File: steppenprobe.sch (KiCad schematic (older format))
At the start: 85 parts, among them J1 USB_C_Receptacle_USB2.0, J2 Conn_ST_STDC14, J4 Conn_01x16, Q1 2N7002, SW1 SW_SPDT, SW2 SW_Push, U1 FT2232HL, U10 74LVC1G125, U11 74LVC1G125, U12 74LVC1G125, U2 XC6206PxxxMR, U3 SRV05-4, U4 93LCxxB, U5 74LVC1G125, U6 74LVC1G126, U7 74LVC1G125, U8 74LVC1G125, U9 74LVC1G125, Y1 Crystal_GND24

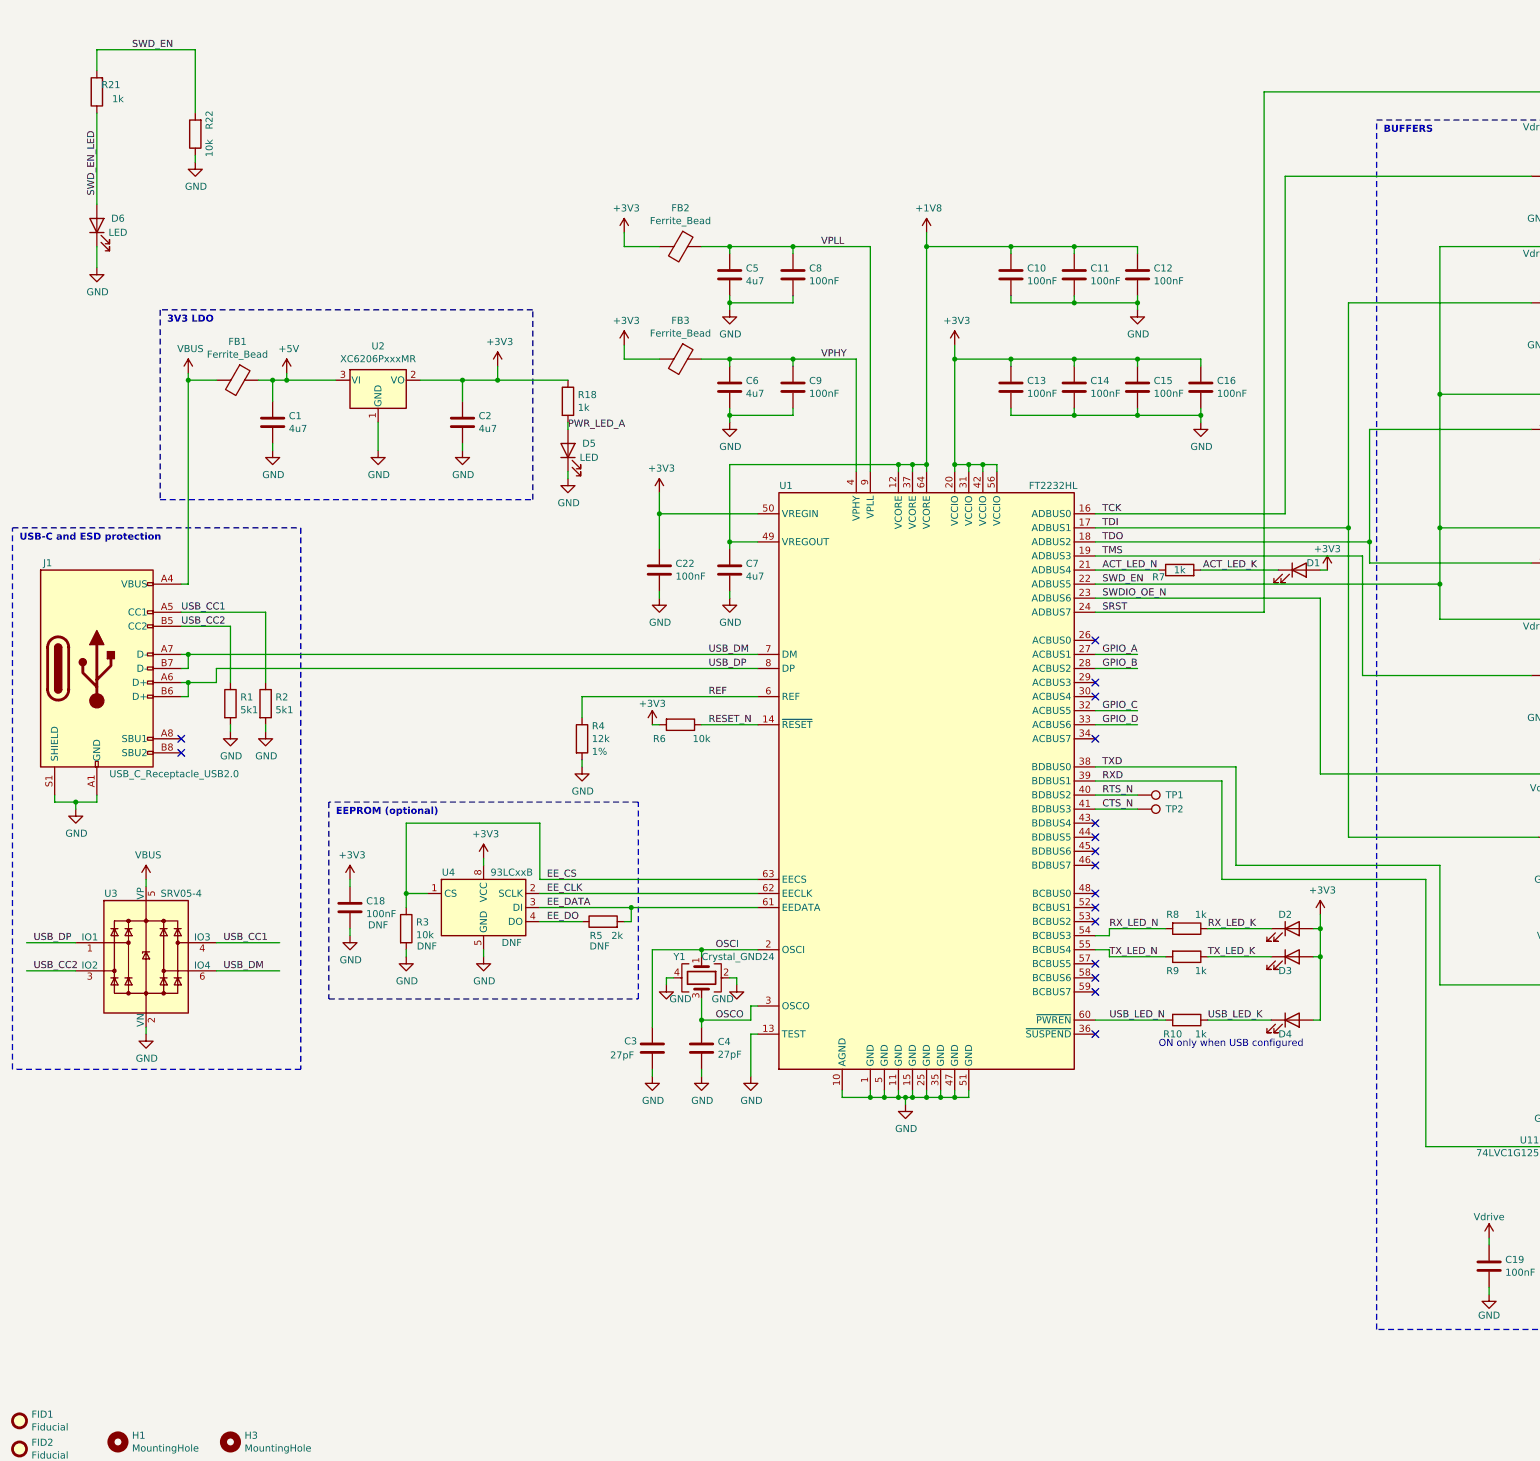
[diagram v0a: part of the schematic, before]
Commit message: Small schematic tidy-up
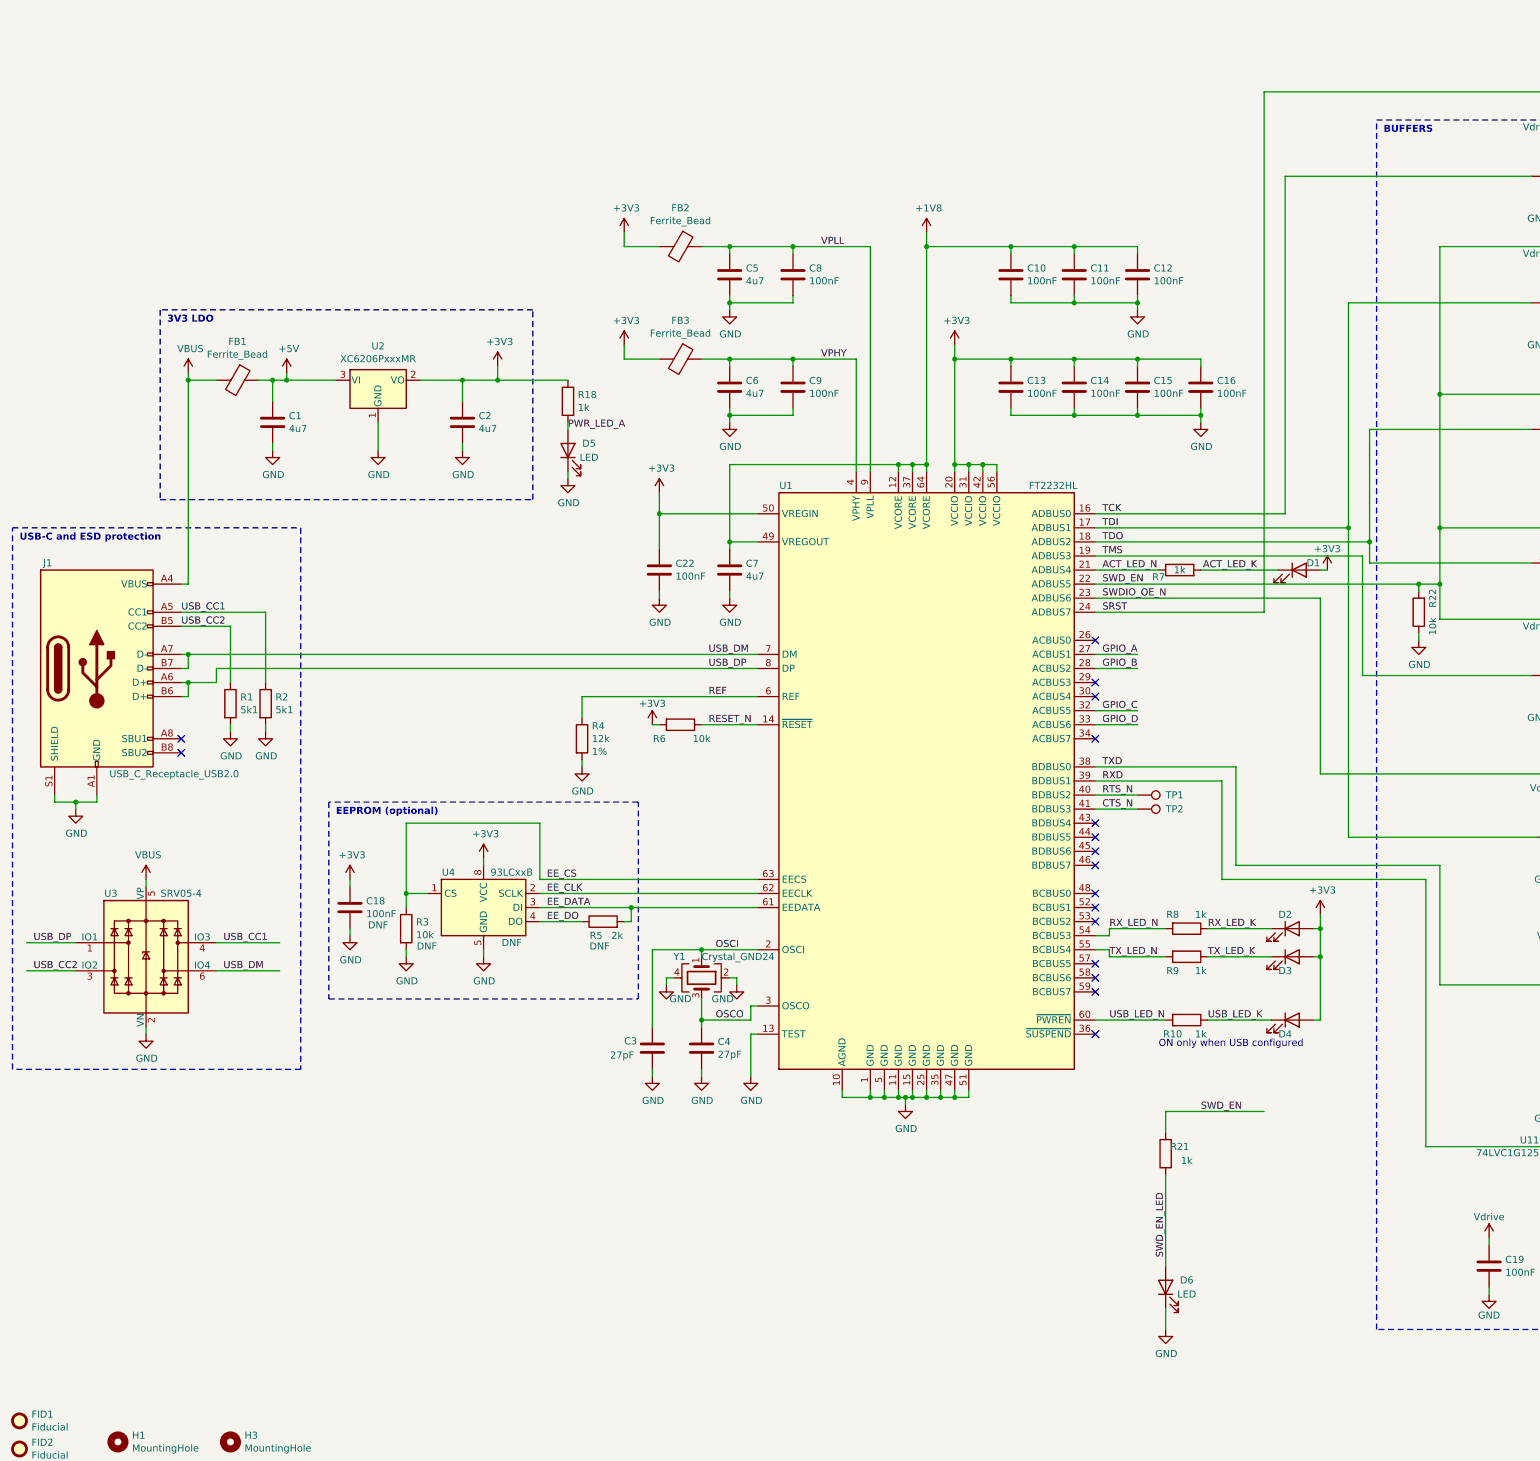
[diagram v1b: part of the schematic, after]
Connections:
- wire segments 373 -> 374
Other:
- moved on the sheet: D6, R21, R22
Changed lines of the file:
@@
 	8400 5950 9300 5950
 Wire Wire Line
-	8400 4550 10850 4550
+	8400 4550 10700 4550
 Wire Wire Line
 	8400 4350 10300 4350
@@
 	11800 4800 10850 4800
 Wire Wire Line
-	10850 4800 10850 4550
-Wire Wire Line
 	11800 4800 11800 5000
 Connection ~ 10850 4550
@@
 L Device:LED D6
 U 1 1 5D606F34
-P 1300 2000
-F 0 "D6" V 1350 1850 50  0000 C CNN
-F 1 "LED" V 1250 1850 50  0000 C CNN
-F 2 "LED_SMD:LED_0603_1608Metric" H 1300 2000 50  0001 C CNN
-F 3 "~" H 1300 2000 50  0001 C CNN
-F 4 "C72043" H 1300 2000 50  0001 C CNN "LCSC_PN"
-F 5 "19-217/GHC-YR1S2/3T" H 1300 2000 50  0001 C CNN "MPN"
-F 6 "Everlight Elec" H 1300 2000 50  0001 C CNN "Manufacturer"
-F 7 "150060GS75000" H 1300 2000 50  0001 C CNN "MPN2"
-F 8 "Wurth Electronic" H 1300 2000 50  0001 C CNN "Manufacturer2"
-	1    1300 2000
+P 8900 9550
+F 0 "D6" V 8950 9400 50  0000 C CNN
+F 1 "LED" V 8850 9400 50  0000 C CNN
+F 2 "LED_SMD:LED_0603_1608Metric" H 8900 9550 50  0001 C CNN
+F 3 "~" H 8900 9550 50  0001 C CNN
+F 4 "C72043" H 8900 9550 50  0001 C CNN "LCSC_PN"
+F 5 "19-217/GHC-YR1S2/3T" H 8900 9550 50  0001 C CNN "MPN"
+F 6 "Everlight Elec" H 8900 9550 50  0001 C CNN "Manufacturer"
+F 7 "150060GS75000" H 8900 9550 50  0001 C CNN "MPN2"
+F 8 "Wurth Electronic" H 8900 9550 50  0001 C CNN "Manufacturer2"
+	1    8900 9550
 	0    -1   -1   0
 $EndComp
@@
 L Device:R R21
 U 1 1 5D606F4F
-P 1300 1050
-F 0 "R21" H 1200 1000 50  0000 C CNN
-F 1 "1k" H 1150 1100 50  0000 C CNN
-F 2 "Resistor_SMD:R_0603_1608Metric" V 1230 1050 50  0001 C CNN
-F 3 "~" H 1300 1050 50  0001 C CNN
-F 4 "C21190" H 1300 1050 50  0001 C CNN "LCSC_PN"
-F 5 "5%" H 1300 1050 50  0001 C CNN "Tolerance"
-	1    1300 1050
+P 8900 8600
+F 0 "R21" H 8800 8550 50  0000 C CNN
+F 1 "1k" H 8750 8650 50  0000 C CNN
+F 2 "Resistor_SMD:R_0603_1608Metric" V 8830 8600 50  0001 C CNN
+F 3 "~" H 8900 8600 50  0001 C CNN
+F 4 "C21190" H 8900 8600 50  0001 C CNN "LCSC_PN"
+F 5 "5%" H 8900 8600 50  0001 C CNN "Tolerance"
+	1    8900 8600
 	-1   0    0    1
 $EndComp
 Wire Wire Line
-	1300 1850 1300 1200
-Wire Wire Line
-	1300 900  1300 750
-Wire Wire Line
-	1300 750  2000 750
-Text Label 1550 750  0    50   ~ 0
+	8900 9400 8900 8750
+Wire Wire Line
+	8900 8450 8900 8300
+Wire Wire Line
+	8900 8300 9600 8300
+Text Label 9150 8300 0    50   ~ 0
 SWD_EN
 $Comp
@@
 L power:GND #PWR0106
 U 1 1 5D606F41
-P 1300 2300
-F 0 "#PWR0106" H 1300 2050 50  0001 C CNN
-F 1 "GND" H 1305 2127 50  0000 C CNN
-F 2 "" H 1300 2300 50  0001 C CNN
-F 3 "" H 1300 2300 50  0001 C CNN
-	1    1300 2300
-	1    0    0    -1
-$EndComp
-Wire Wire Line
-	1300 2150 1300 2300
-Text Label 1300 1325 3    50   ~ 0
+P 8900 9850
+F 0 "#PWR0106" H 8900 9600 50  0001 C CNN
+F 1 "GND" H 8905 9677 50  0000 C CNN
+F 2 "" H 8900 9850 50  0001 C CNN
+F 3 "" H 8900 9850 50  0001 C CNN
+	1    8900 9850
+	1    0    0    -1
+$EndComp
+Wire Wire Line
+	8900 9700 8900 9850
+Text Label 8900 8875 3    50   ~ 0
 SWD_EN_LED
 $Comp
@@
 	1    0    0    -1
 $EndComp
-$Comp
-L Device:R R22
-U 1 1 5DF52301
-P 2000 1350
-F 0 "R22" V 1900 1250 50  0000 C CNN
-F 1 "10k" V 1900 1450 50  0000 C CNN
-F 2 "Resistor_SMD:R_0603_1608Metric" V 1930 1350 50  0001 C CNN
-F 3 "~" H 2000 1350 50  0001 C CNN
-F 4 "C25804" H 2000 1350 50  0001 C CNN "LCSC_PN"
-F 5 "5%" H 2000 1350 50  0001 C CNN "Tolerance"
-	1    2000 1350
-	-1   0    0    1
-$EndComp
-Wire Wire Line
-	2000 1500 2000 1550
-$Comp
-L power:GND #PWR065
-U 1 1 5DF533AF
-P 2000 1550
-F 0 "#PWR065" H 2000 1300 50  0001 C CNN
-F 1 "GND" H 2005 1377 50  0000 C CNN
-F 2 "" H 2000 1550 50  0001 C CNN
-F 3 "" H 2000 1550 50  0001 C CNN
-	1    2000 1550
-	1    0    0    -1
-$EndComp
-Wire Wire Line
-	2000 1200 2000 750
 Wire Wire Line
 	13850 1450 13850 1650
@@
 	1    0    0    -1
 $EndComp
+Wire Wire Line
+	10850 4800 10850 4550
+Wire Wire Line
+	10700 4900 10700 4950
+$Comp
+L power:GND #PWR065
+U 1 1 5DF533AF
+P 10700 4950
+F 0 "#PWR065" H 10700 4700 50  0001 C CNN
+F 1 "GND" H 10705 4777 50  0000 C CNN
+F 2 "" H 10700 4950 50  0001 C CNN
+F 3 "" H 10700 4950 50  0001 C CNN
+	1    10700 4950
+	1    0    0    -1
+$EndComp
+$Comp
+L Device:R R22
+U 1 1 5DF52301
+P 10700 4750
+F 0 "R22" V 10600 4650 50  0000 C CNN
+F 1 "10k" V 10600 4850 50  0000 C CNN
+F 2 "Resistor_SMD:R_0603_1608Metric" V 10630 4750 50  0001 C CNN
+F 3 "~" H 10700 4750 50  0001 C CNN
+F 4 "C25804" H 10700 4750 50  0001 C CNN "LCSC_PN"
+F 5 "5%" H 10700 4750 50  0001 C CNN "Tolerance"
+	1    10700 4750
+	-1   0    0    1
+$EndComp
+Wire Wire Line
+	10700 4600 10700 4550
+Connection ~ 10700 4550
+Wire Wire Line
+	10700 4550 10850 4550
 $EndSCHEMATC
